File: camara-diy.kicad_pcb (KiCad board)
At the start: 2 copper layers, 59.5 x 47 mm, 19 parts, among them J1 Conn_01x07, J3 Conn_01x02, SW1 SW_Push, SW2 SW_Push, U1 XIAO-ESP32-S3-SMD, U2 TP4056-42-ESOP8

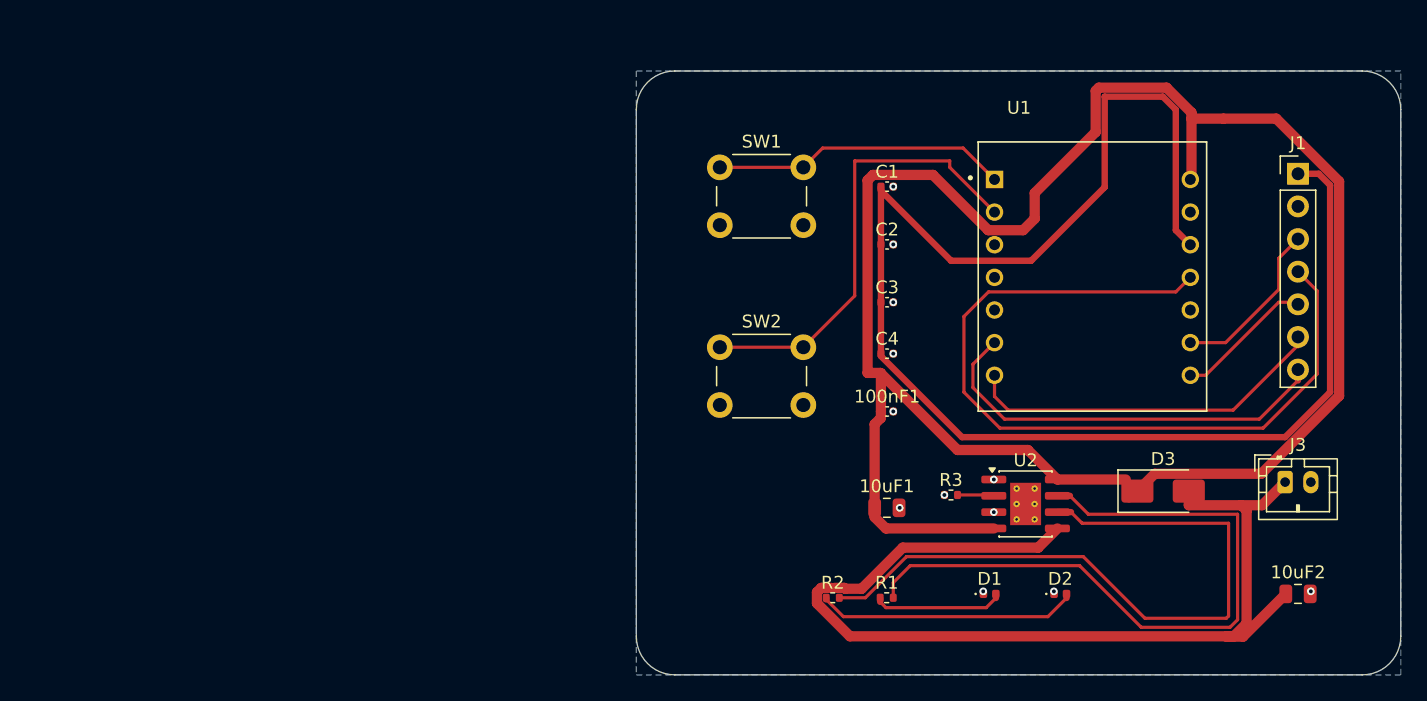
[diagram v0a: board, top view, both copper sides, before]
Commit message: archivos actualizados + assets de componentes
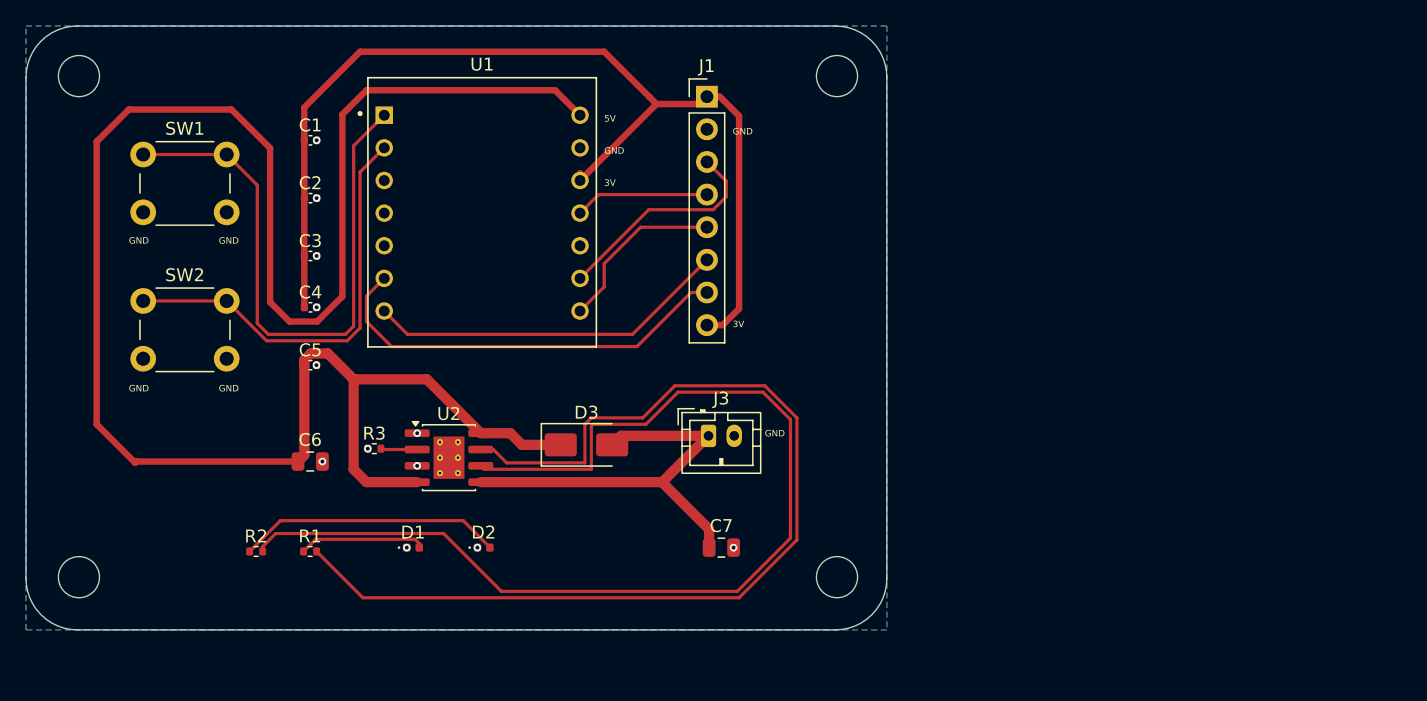
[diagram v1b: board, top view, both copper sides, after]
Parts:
- added REF**: MountingHole_3.2mm_M3, MountingHole:MountingHole_3.2mm_M3, F.Cu at (170.6, 124.9)
- added REF**: MountingHole_3.2mm_M3, MountingHole:MountingHole_3.2mm_M3, F.Cu at (111.6, 85.9)
- added REF**: MountingHole_3.2mm_M3, MountingHole:MountingHole_3.2mm_M3, F.Cu at (111.6, 124.9)
- added REF**: MountingHole_3.2mm_M3, MountingHole:MountingHole_3.2mm_M3, F.Cu at (170.6, 85.9)
- C1, C2, C3, C4: value C -> 100nF
- C5: renamed from 100nF1; value C5 -> 100nF
- C6: renamed from 10uF1; value C6 -> 10uF
- C7: renamed from 10uF2; value C7 -> 10uF
- D1: value LED -> LED rojo
- D2: value LED -> LED verde
- D3: value D_Schottky -> D_Schottky SS14
- J1: value Conn_01x07 -> GC9A01_8P; footprint Connector_PinHeader_2.54mm:PinHeader_1x07_P2.54mm_Vertical -> Connector_PinHeader_2.54mm:PinHeader_1x08_P2.54mm_Vertical
- J3: value Conn_01x02 -> Batería 18650
- R1, R2: value R -> 1k
- SW1: value SW_Push -> Shutter
- SW2: value SW_Push -> Modo
- moved U1 47.8 mm to (143.0, 96.5)
- moved J1 46.4 mm to (160.5, 87.5)
- moved C1 45.0 mm to (129.6, 90.9)
- moved C2 45.0 mm to (129.6, 95.4)
- moved C3 45.0 mm to (129.6, 99.9)
- moved C4 45.0 mm to (129.6, 103.9)
- moved C5 45.0 mm to (129.6, 108.4)
- moved U2 45.0 mm to (140.4, 115.6)
- moved C6 45.0 mm to (129.6, 115.9)
- moved C7 45.0 mm to (161.6, 122.6)
- moved D1 45.0 mm to (137.6, 122.6)
- moved D2 45.0 mm to (143.1, 122.6)
- moved D3 45.0 mm to (151.1, 114.6)
- moved J3 45.0 mm to (160.6, 113.9)
- moved R1 45.0 mm to (129.6, 122.9)
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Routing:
- net /SPI_MOSI: track 63.8 -> 10.5 mm
- net /BAT_18650: track 81.5 -> 33.6 mm
- net +3V3: track 117.5 -> 80.8 mm
- net Net-(U2-~{STDBY}): track 54.6 -> 84.2 mm
- net Net-(U2-~{CHRG}): track 53.6 -> 80.5 mm
- net /BTN_SHUTTER: track 23.0 -> 46.1 mm
- net /SPI_CLK: track 13.1 -> 17.3 mm
- net /DISP_RES: track 10.8 -> 13.6 mm
- net /BTN_MODO: track 35.5 -> 33.4 mm
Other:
- board size 59.5 x 47 mm -> 67 x 47 mm
- board text added: "3V"
- board text added: "5V"
- board text added: "GND"
